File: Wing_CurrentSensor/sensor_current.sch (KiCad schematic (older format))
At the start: 20 parts, among them J1 feather long, J2 feather short, J3 SJ-3524-SMT, J4 Analog Selection, U1 TL084, U2 AD8226

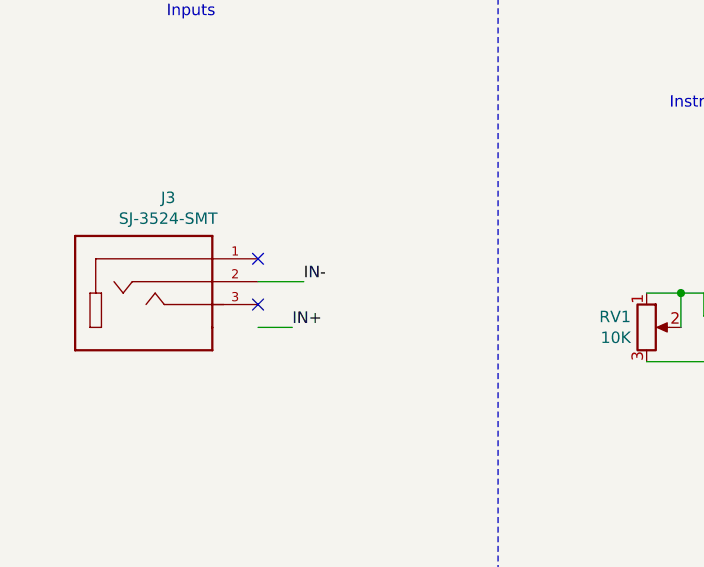
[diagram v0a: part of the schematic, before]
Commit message: Add_Connector
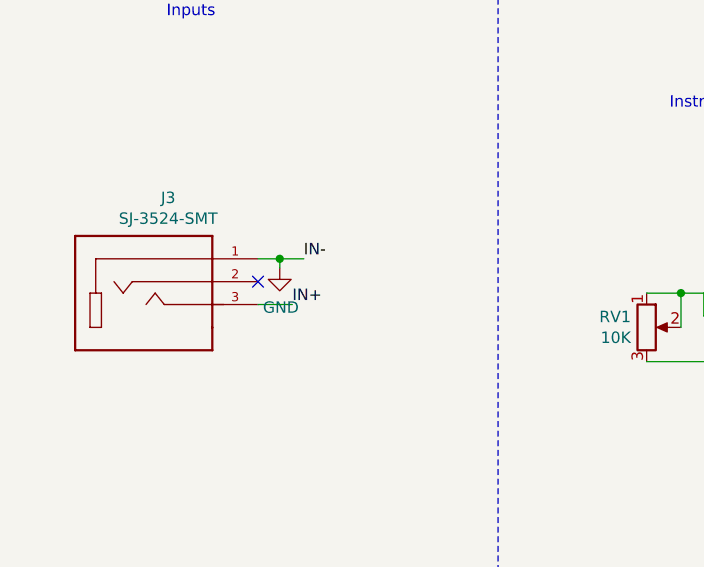
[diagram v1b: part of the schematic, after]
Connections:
- net GND: now also J3.1, U2.1 (-)
- net IN+: now also J3.3
- net IN-: no longer names the net of J3.2
- net IN-: no longer U2.1 (-)
- no-connect marks 22 -> 21
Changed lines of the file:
@@
 Wire Wire Line
 	8400 4100 9250 4100
-Text Label 1650 2000 0    50   ~ 0
+Text Label 1650 1900 0    50   ~ 0
 IN+
-Text Label 1700 1800 0    50   ~ 0
+Text Label 1700 1700 0    50   ~ 0
 IN-
 NoConn ~ 10050 5000
@@
 $EndComp
 Wire Wire Line
-	1500 1800 1700 1800
-Wire Wire Line
-	1500 2000 1650 2000
+	1500 1700 1595 1700
+Wire Wire Line
+	1500 1900 1650 1900
 NoConn ~ 10300 4900
 NoConn ~ 10300 4800
@@
 	1    0    0    -1
 $EndComp
-NoConn ~ 1500 1900
-NoConn ~ 1500 1700
+NoConn ~ 1500 1800
 NoConn ~ 9050 4800
 NoConn ~ 9050 4900
@@
 	1    0    0    -1
 $EndComp
+$Comp
+L power:GND #PWR0108
+U 1 1 60D403E1
+P 1595 1740
+F 0 "#PWR0108" H 1595 1490 50  0001 C CNN
+F 1 "GND" H 1600 1567 50  0000 C CNN
+F 2 "" H 1595 1740 50  0001 C CNN
+F 3 "" H 1595 1740 50  0001 C CNN
+	1    1595 1740
+	1    0    0    -1
+$EndComp
+Wire Wire Line
+	1595 1740 1595 1700
+Connection ~ 1595 1700
+Wire Wire Line
+	1595 1700 1700 1700
 $EndSCHEMATC

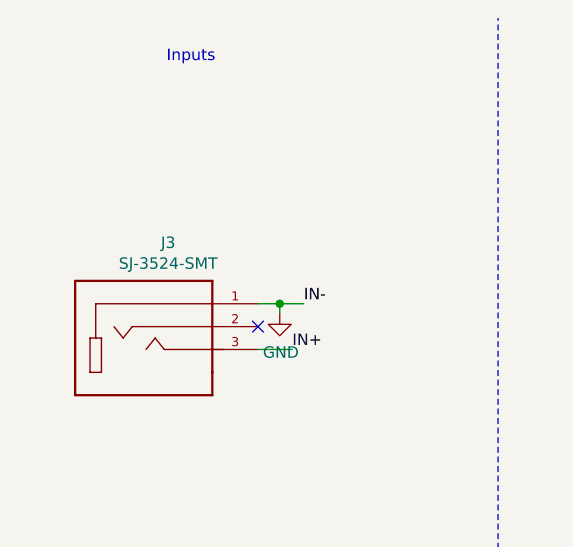
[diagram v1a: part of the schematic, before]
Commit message: Change_BOM
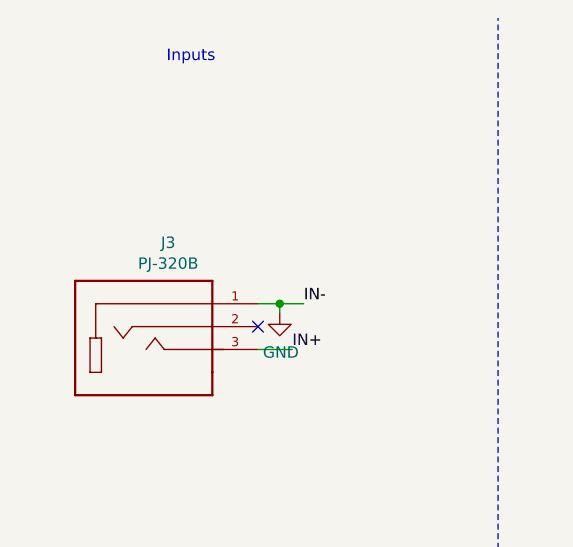
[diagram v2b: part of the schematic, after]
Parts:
- J3: value SJ-3524-SMT -> PJ-320B
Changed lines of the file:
@@
 P 1000 1900
 F 0 "J3" H 1107 2367 50  0000 C CNN
-F 1 "SJ-3524-SMT" H 1107 2276 50  0000 C CNN
+F 1 "PJ-320B" H 1107 2276 50  0000 C CNN
 F 2 "CUI_SJ-3524-SMT" H 1000 1900 50  0001 L BNN
 F 3 "" H 1000 1900 50  0001 L BNN
